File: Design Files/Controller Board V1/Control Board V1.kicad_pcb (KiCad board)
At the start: 4 copper layers, 75 x 125 mm, 72 parts, among them J1 XT30PW-F, J10 SM04B-GHS-TB_LF__SN_-, J11 SM04B-GHS-TB_LF__SN_-, J2 XT30UPB-M, J3 XT30UPB-M, J4 XT30UPB-M, J5 XT30UPB-M, J6 XT30UPB-M, J7 XT30UPB-M, J8 SM04B-GHS-TB_LF__SN_-, J9 SM04B-GHS-TB_LF__SN_-, Q1 LMG5200, U1 LMR51420XDDCR, U2 INA219BIDR, U3 INA219BIDR, U4 INA219BIDR, U5 SC0917

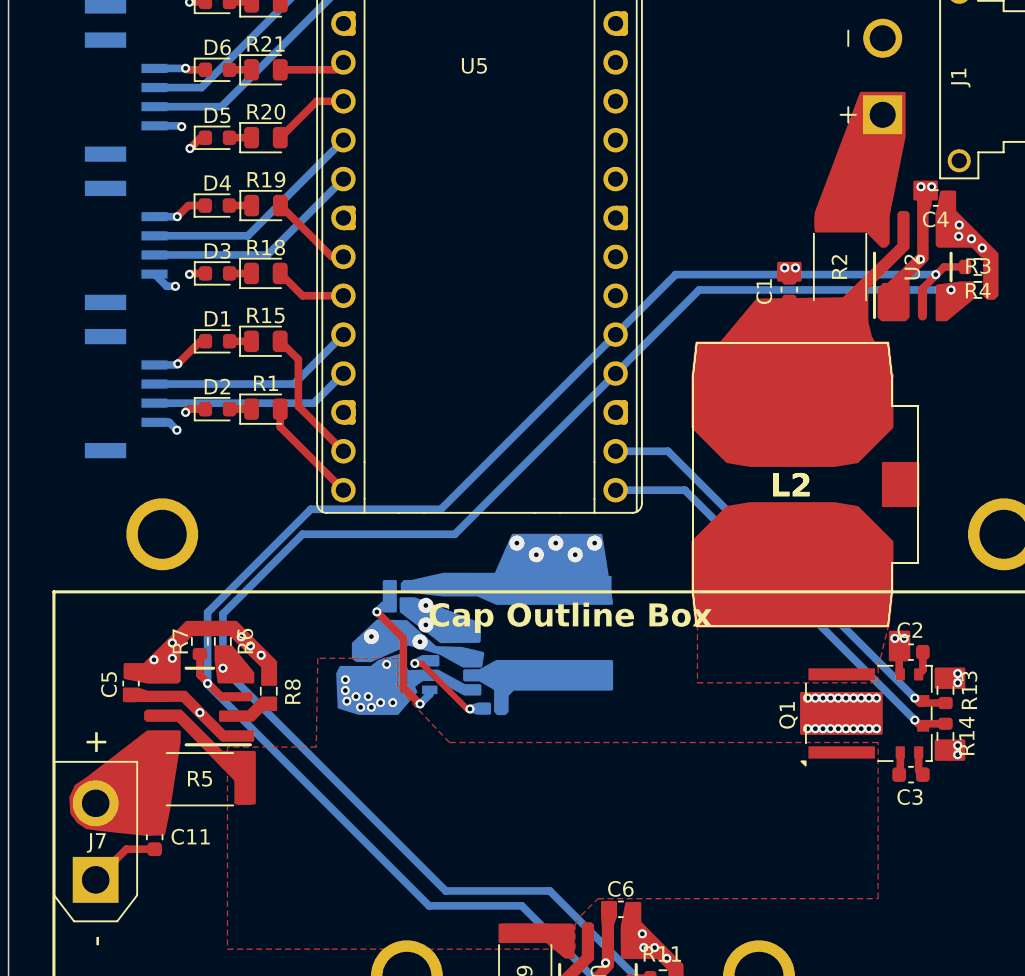
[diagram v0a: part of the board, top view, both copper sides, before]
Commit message: finished the stuffs
yippee
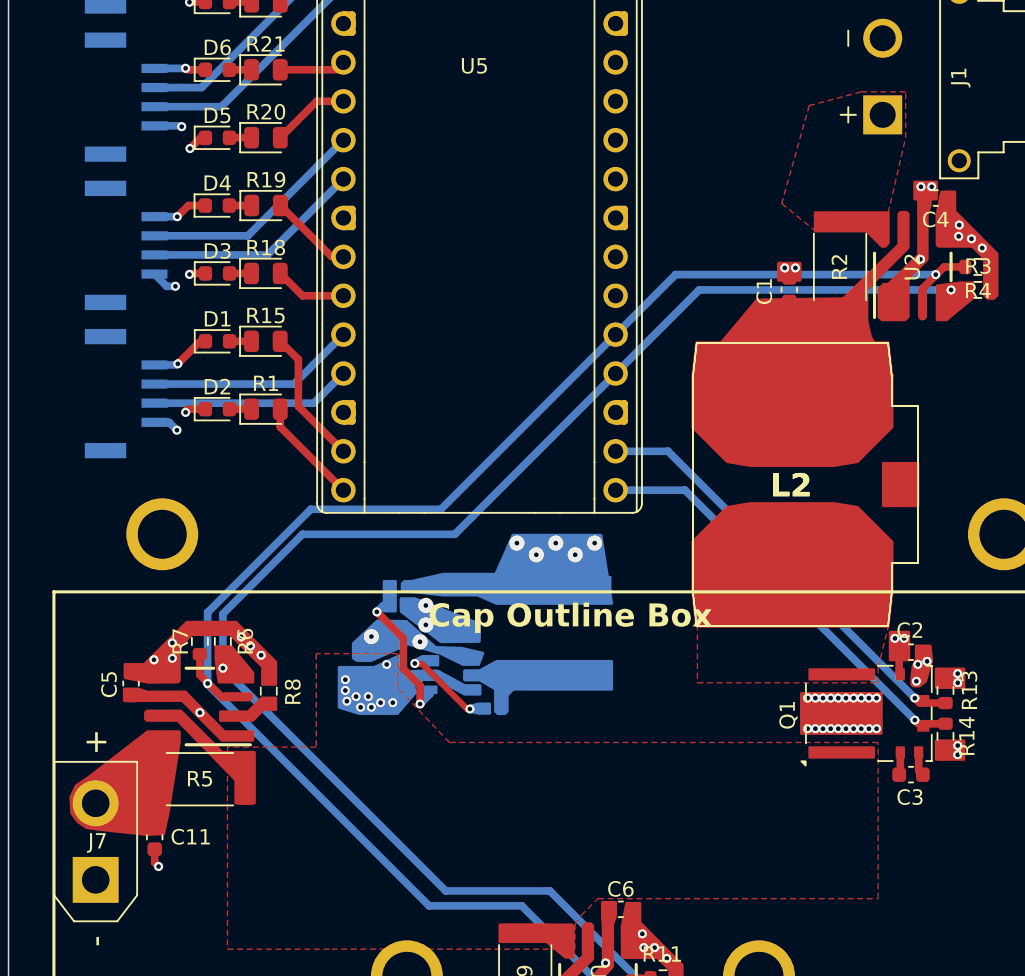
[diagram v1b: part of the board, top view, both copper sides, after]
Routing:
- net P_GND: track 33.7 -> 30.3 mm, vias 50 -> 51
- net 5V: track 7.37 -> 5.81 mm, vias 22 -> 25
- added copper zone on F.Cu, net /CAP_IN
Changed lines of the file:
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@@
 	(gr_poly
 		(pts
-			(xy 115.260877 75.183181) (xy 118.560877 75.183181) (xy 119.560877 76.183181) (xy 119.760877 76.183181)
-			(xy 119.960877 75.983181) (xy 119.960877 74.183181) (xy 121 69) (xy 121 66.2) (xy 118.2 66.2) (xy 115.260877 73.983181)
+			(xy 115.2 75.183181) (xy 118.560877 75.183181) (xy 119.560877 76.183181) (xy 119.760877 76.183181)
+			(xy 119.960877 75.983181) (xy 119.960877 74) (xy 115.2 74)
 		)
 		(stroke
@@
 		(fill none)
 		(layer "F.Cu")
+	)
+	(gr_poly
+		(pts
+			(xy 121.6 104.9) (xy 121.5 104.8) (xy 121.5 104.4) (xy 121.6 103.6) (xy 121.8 103.2) (xy 121.8 102.3)
+			(xy 122.7 102.3) (xy 122.8 103.3) (xy 122.7 103.5) (xy 122.4 104.6) (xy 122 104.9)
+		)
+		(stroke
+			(width 0.2)
+			(type solid)
+		)
+		(fill solid)
+		(layer "F.Cu")
+		(net 6)
 	)
 	(gr_poly
@@
 	(gr_poly
 		(pts
-			(xy 85.026398 102.139369) (xy 86.597851 100.667569) (xy 88.488581 100.708877) (xy 90.4 102.4) (xy 92.114482 102.455667)
-			(xy 93.473914 102.775615) (xy 93.351264 103.603502) (xy 92.201421 103.603502) (xy 90.706625 102.775616)
-			(xy 88.606244 102.162365) (xy 86.176242 103.250884) (xy 85.23337 103.235553) (xy 85.026398 103.074574)
+			(xy 85.024977 102.135867) (xy 86.59643 100.664067) (xy 88.48716 100.705375) (xy 90.398579 102.396498)
+			(xy 92.113061 102.452165) (xy 93.472493 102.772113) (xy 93.198579 103.496498) (xy 92.2 103.5) (xy 90.705204 102.772114)
+			(xy 88.604823 102.158863) (xy 86.174821 103.247382) (xy 85.231949 103.232051) (xy 85.024977 103.071072)
 		)
 		(stroke
@@
 	(gr_poly
 		(pts
-			(xy 84 104.1) (xy 84.1 106.3) (xy 85.4 106.7) (xy 87.9 106.7) (xy 89.1 105.3) (xy 88.1 102.9) (xy 86.7 103.3)
-			(xy 86.2 103.7) (xy 84.2 103.7)
+			(xy 84.1 106.3) (xy 85.4 106.7) (xy 87.9 106.7) (xy 89.1 105.3) (xy 88.1 102.9) (xy 86.4 103.7) (xy 84.1 103.7)
 		)
 		(stroke
@@
 	)
 	(segment
+		(start 72.045828 115.57)
+		(end 72.045828 116.445828)
+		(width 0.5)
+		(layer "F.Cu")
+		(net 4)
+	)
+	(segment
 		(start 75.36275 77.959613)
 		(end 74.384167 77.959613)
@@
 	)
 	(segment
-		(start 72.045828 115.57)
-		(end 70.194171 115.57)
-		(width 0.5)
-		(layer "F.Cu")
-		(net 4)
-	)
-	(segment
 		(start 85.933334 155.375)
 		(end 85.933334 156.133334)
@@
 	)
 	(segment
+		(start 72.045828 116.445828)
+		(end 72.3 116.7)
+		(width 0.5)
+		(layer "F.Cu")
+		(net 4)
+	)
+	(segment
 		(start 114.070167 156.070167)
 		(end 114.4 156.4)
@@
 	)
 	(segment
-		(start 70.194171 115.57)
-		(end 68.191643 117.572528)
-		(width 0.5)
-		(layer "F.Cu")
-		(net 4)
-	)
-	(segment
 		(start 120.675 104.075)
 		(end 120.75 104.15)
@@
 	)
 	(via blind
+		(at 72.3 116.7)
+		(size 0.6)
+		(drill 0.3)
+		(layers "F.Cu" "In1.Cu")
+		(net 4)
+	)
+	(via blind
 		(at 73.504631 57.396411)
 		(size 0.6)
@@
 		(net 5)
 	)
-	(segment
-		(start 122.225 103.875)
-		(end 121.95 104.15)
-		(width 0.5)
-		(layer "F.Cu")
-		(net 6)
-	)
-	(segment
-		(start 122.225 102.7)
-		(end 122.225 103.875)
-		(width 0.5)
-		(layer "F.Cu")
-		(net 6)
-	)
 	(via blind
 		(at 79 102.9)
@@
 	)
 	(via blind
+		(at 121.9 103.5)
+		(size 0.6)
+		(drill 0.3)
+		(layers "F.Cu" "In2.Cu")
+		(free yes)
+		(net 6)
+	)
+	(via blind
 		(at 125.4 75.7)
 		(size 0.6)
@@
 	)
 	(via blind
+		(at 121.8 104.6)
+		(size 0.6)
+		(drill 0.3)
+		(layers "F.Cu" "In2.Cu")
+		(free yes)
+		(net 6)
+	)
+	(via blind
 		(at 126.1 76.3)
+		(size 0.6)
+		(drill 0.3)
+		(layers "F.Cu" "In2.Cu")
+		(free yes)
+		(net 6)
+	)
+	(via blind
+		(at 122.5 103.3)
 		(size 0.6)
 		(drill 0.3)
@@
 	)
 	(segment
-		(start 88.288929 104.994196)
+		(start 89.379778 104.879778)
+		(end 88.288929 103.788929)
+		(width 0.5)
+		(layer "F.Cu")
+		(net 28)
+	)
+	(segment
+		(start 88.288929 103.788929)
 		(end 88.288929 101.79877)
 		(width 0.5)
@@
 	(segment
 		(start 89.379778 106.085045)
-		(end 88.288929 104.994196)
+		(end 89.379778 104.879778)
 		(width 0.5)
 		(layer "F.Cu")
@@
 			(pts
 				(xy 76.8 108.9) (xy 76.8 113.3) (xy 76.8 122.1) (xy 83.6 122.1) (xy 99.5 122.1) (xy 99.5 120.5)
-				(xy 99.9 119.9) (xy 101 118.8) (xy 119.3 118.8) (xy 119.3 108.6) (xy 91.3 108.6) (xy 87.9 105) (xy 87.9 103.1)
-				(xy 85.1 103.1) (xy 82.7 103.1) (xy 82.6 108.9)
+				(xy 99.9 119.9) (xy 101 118.8) (xy 119.3 118.8) (xy 119.3 108.6) (xy 91.3 108.6) (xy 87.9 105) (xy 87.9 102.8)
+				(xy 82.6 102.8) (xy 82.6 108.9)
 			)
 		)
@@
 	)
 	(zone
+		(net 7)
+		(net_name "/CAP_IN")
+		(layer "F.Cu")
+		(hatch none 0.5)
+		(priority 1)
+		(connect_pads yes
+			(clearance 0)
+		)
+		(min_thickness 0.25)
+		(filled_areas_thickness no)
+		(fill yes
+			(thermal_gap 0.5)
+			(thermal_bridge_width 0.5)
+			(island_removal_mode 1)
+			(island_area_min 10)
+		)
+		(polygon
+			(pts
+				(xy 115.2 75.183181) (xy 119.960877 74) (xy 121.1 69.1) (xy 121.1 66.1) (xy 118.2 66.1) (xy 114.8 67)
+				(xy 113 73.4)
+			)
+		)
+	)
+	(zone
 		(net 4)
 		(net_name "P_GND")
@@
 		(polygon
 			(pts
-				(xy 123 101.5) (xy 123.5 103.2) (xy 122.4 105) (xy 108 105) (xy 108 101.5)
+				(xy 122.8 101.5) (xy 123.5 103.2) (xy 122.8 105) (xy 108 105) (xy 108 101.5)
 			)
 		)
@@
 			"583f4df7-8fac-4cbd-82ce-f205a44a597c" "5d9e4cb1-e675-4766-86f6-c9fbc5cd8f8f"
 			"5e24a0d1-ffb5-4ccc-8d19-4f8c13946d0e" "5e960d50-e155-412f-96fc-e3142376b7e8"
-			"68d7e094-cd08-4d67-b0e3-78303260dc1e" "6cf498db-3432-45d3-8c32-362254403798"
+			"640729bb-d87d-45f8-bb5f-7fb30d67480c" "6cf498db-3432-45d3-8c32-362254403798"
 			"6fcb1b68-7ee1-4a5c-99de-65e6fa297009" "7524d766-485d-4db8-82db-5c5d20982b83"
 			"76bea91c-fd3f-49b3-8351-fa2908513b24" "79fb91fa-d631-46f4-a465-6aafe271f5f5"
-			"8b0a0997-ac0a-4843-9d3c-7aba647cdfc4" "97e8f3d6-9ae4-49f6-9d14-747fa14f0a50"
+			"7f770451-475f-427e-a839-d25e019b1486" "8b0a0997-ac0a-4843-9d3c-7aba647cdfc4"
+			"94de7636-d79e-4243-8107-30afec6cb93c" "97e8f3d6-9ae4-49f6-9d14-747fa14f0a50"
 			"9b16b59e-c7ed-471c-910c-8daa297b2831" "9cac112b-d2e7-4d06-8906-c0670bea4c48"
 			"a3925c4d-db26-45a8-88d8-d9c2b1d4682e" "a7862c28-294d-4fba-864e-b5acfd495a3a"
 			"a9f3f0e8-963c-4c59-be1b-b4fcc45b154f" "abc72818-2439-4c0e-8367-a4768fb89b16"
-			"b2158cf1-eb62-44fc-acc6-f40ad1d21d73" "bded6fd2-167c-4a3c-b67c-34651a94f9e5"
+			"b2158cf1-eb62-44fc-acc6-f40ad1d21d73" "be421fbe-92af-480e-a00a-106512b46463"
 			"c198362b-c47e-4b00-a246-c995cf1e92e2" "c75d7a87-7e86-44d0-86e0-ba194b234927"
 			"cbc1f7fa-b2af-4bee-b431-f5128f3fc790" "ce336664-c232-4bd1-8327-4e3bc8ae5cfa"
@@
 			"330b5346-ee03-4ccb-a2e8-f70af065349e" "362cf553-4c6f-44a3-814f-9aafacb7149e"
 			"3786135e-dc1e-46f8-adb4-22b06da3b455" "37a72350-153e-4021-9f44-709499478770"
-			"37ac942c-c820-4023-ac99-d4c7229de39a" "3943b47c-c5f9-4d98-839c-defade32b3d6"
-			"3a7ffc72-b672-41e5-9450-376bbc01c79b" "46a726ba-56ee-4520-b2d3-d4d7cdf6566b"
-			"526b88f3-1dab-422e-893f-1b2c01fe874f" "546cac1f-572f-49ff-8702-6f9544b5b6f2"
-			"5c8aaf3b-7e70-4f96-a209-0fc7e1262841" "62601344-9b4f-4d08-9275-5624dfc40f33"
-			"62b2ec5d-2978-4c0b-a0d9-f369fb6edd4d" "66176771-d532-460d-93e4-c4fcde17ff9b"
-			"6632844a-c0a0-48b9-bddc-6fd729e13e40" "681d5738-adf9-4486-84c9-fdf01cff44b9"
-			"69719426-1875-4073-a496-a9386f5beb8f" "6d70b5e3-2cca-49e6-a7e6-5546aec6c352"
-			"735188d5-e988-40c1-8d32-c965199fea6d" "74bf968a-2eb9-4f31-815a-4a151dd0e82c"
-			"7740900c-165d-4e62-abd3-4689b696aaf7" "7b525c96-2723-4a41-9cee-f33cf8efd5d7"
+			"3943b47c-c5f9-4d98-839c-defade32b3d6" "3a7ffc72-b672-41e5-9450-376bbc01c79b"
+			"46a726ba-56ee-4520-b2d3-d4d7cdf6566b" "526b88f3-1dab-422e-893f-1b2c01fe874f"
+			"546cac1f-572f-49ff-8702-6f9544b5b6f2" "5c8aaf3b-7e70-4f96-a209-0fc7e1262841"
+			"62601344-9b4f-4d08-9275-5624dfc40f33" "62b2ec5d-2978-4c0b-a0d9-f369fb6edd4d"
+			"66176771-d532-460d-93e4-c4fcde17ff9b" "6632844a-c0a0-48b9-bddc-6fd729e13e40"
+			"681d5738-adf9-4486-84c9-fdf01cff44b9" "69719426-1875-4073-a496-a9386f5beb8f"
+			"6d70b5e3-2cca-49e6-a7e6-5546aec6c352" "735188d5-e988-40c1-8d32-c965199fea6d"
+			"74bf968a-2eb9-4f31-815a-4a151dd0e82c" "7740900c-165d-4e62-abd3-4689b696aaf7"
+			"7b525c96-2723-4a41-9cee-f33cf8efd5d7" "852520d6-c01d-43c5-833f-3cd822acd1ff"
 			"91e29a2a-0354-4217-9fe5-f18d4fc59a33" "929ccb9c-92e4-48f6-b01b-3d6677283a92"
-			"930d19a7-7ff0-43f8-81db-066a22cfd5d8" "9964af3c-70ab-4abc-a192-2d251fe86dcc"
-			"9c4b813d-05e7-4548-99e3-6bd1e0cfc629" "add65acd-046f-4b91-86c8-98b1c4fdc4e6"
-			"b511fa1b-357b-4564-84c1-3b721654b8a4" "bafa75cc-7183-468d-bc32-5838b034c9e0"
-			"bd9d6ae3-a2b4-44e1-8bc5-4617d19f2927" "c0a86e8a-b530-47ee-adc4-3694f0d68c0c"
+			"9964af3c-70ab-4abc-a192-2d251fe86dcc" "9da1f060-4254-4a97-a122-ef85e1ae045d"
+			"add65acd-046f-4b91-86c8-98b1c4fdc4e6" "b511fa1b-357b-4564-84c1-3b721654b8a4"
+			"bafa75cc-7183-468d-bc32-5838b034c9e0" "bd9d6ae3-a2b4-44e1-8bc5-4617d19f2927"
+			"c0a86e8a-b530-47ee-adc4-3694f0d68c0c" "c64881d7-e3d4-458c-9106-d891b6cdeaca"
 			"ca964e1e-3cbf-4d6f-ab18-995f1eb3b613" "cb251945-bc11-4f8c-b3d5-1a0f0acfe6df"
-			"d557426c-c26f-4910-9769-4f95ad23c57a" "d931bb5b-1f4b-4898-9407-32404f2cc3c5"
-			"dd631645-3c7b-411d-a646-2cce025b4d8e" "ea4476a5-22ed-4662-be9f-8f747a3393b9"
-			"fa4dea38-8a01-4e5f-a42f-c25cac921510" "fda227e2-c579-4f73-88de-f4c77bf80f8c"
-			"fec5a4e1-a340-4ce4-a8c0-8198ab5b11f2"
-		)
-	)
+			"d557426c-c26f-4910-9769-4f95ad23c57a" "d7c146f3-868d-4ef2-9568-6037358f73d9"
+			"d931bb5b-1f4b-4898-9407-32404f2cc3c5" "dd631645-3c7b-411d-a646-2cce025b4d8e"
+			"ea4476a5-22ed-4662-be9f-8f747a3393b9" "fa4dea38-8a01-4e5f-a42f-c25cac921510"
+			"fda227e2-c579-4f73-88de-f4c77bf80f8c" "fec5a4e1-a340-4ce4-a8c0-8198ab5b11f2"
+		)
+	)
